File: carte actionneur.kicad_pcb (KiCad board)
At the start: 2 copper layers, 108 x 138 mm, 88 parts, among them J1 Conn_01x03_Pin, J10 Conn_01x03_Pin, J11 Conn_01x02, J12 Conn_01x02_Pin, J13 Conn_01x02_Pin, J14 Conn_01x02_Pin, J15 Conn_01x02, J16 Conn_01x02_Pin, J17 Conn_01x04_Pin, J18 Conn_01x02_Pin, J19 Conn_01x04_Pin, J2 Conn_01x02, J20 Conn_01x02_Pin, J21 Conn_01x08_Pin, J22 Conn_01x02_Pin, J23 Conn_01x02_Pin, J24 Conn_01x02_Pin, J25 Conn_01x03_Pin, J26 Conn_01x03_Pin, J27 Conn_01x03_Pin, J28 Conn_01x02_Pin, J3 Conn_01x04_Pin, J4 Conn_01x02_Pin, J5 Connecteur Programmation, J6 Conn_01x08_Pin, J7 Conn_01x03_Pin, J8 Conn_01x03_Pin, J9 Conn_01x03_Pin, Q1 Q_NMOS_GDS, Q2 QM6006D, Q3 QM6006D, Q4 QM6006D, U1 MEGA_PRO_EMBED_CH340G___ATMEG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, U2 YAAJ_DCDC_StepDown_LM2596, U3 ZXBM5210-SP, U4 YAAJ_DCDC_StepDown_LM2596, U5 YAAJ_DCDC_StepDown_LM2596, U7 ZXBM5210-SP

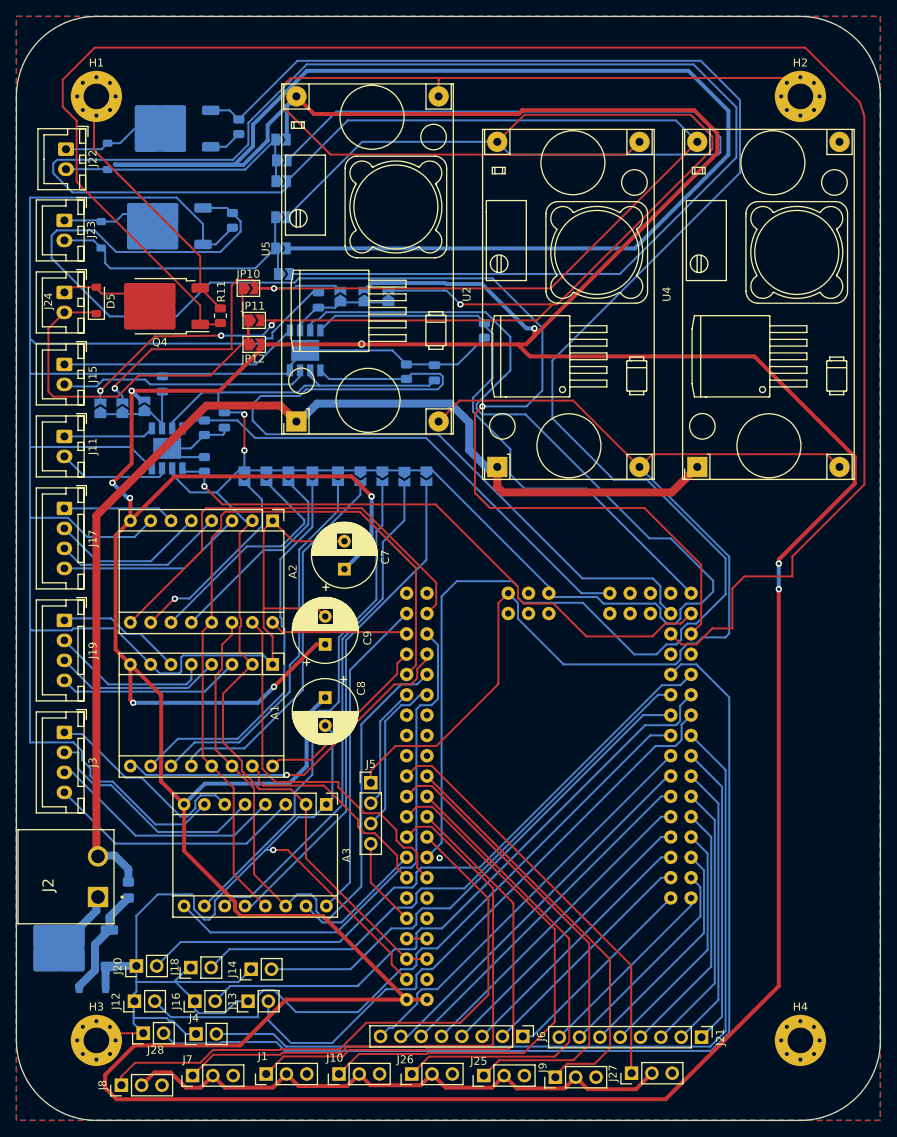
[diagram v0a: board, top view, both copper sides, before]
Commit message: Updated Arduino for 2025 (#1)
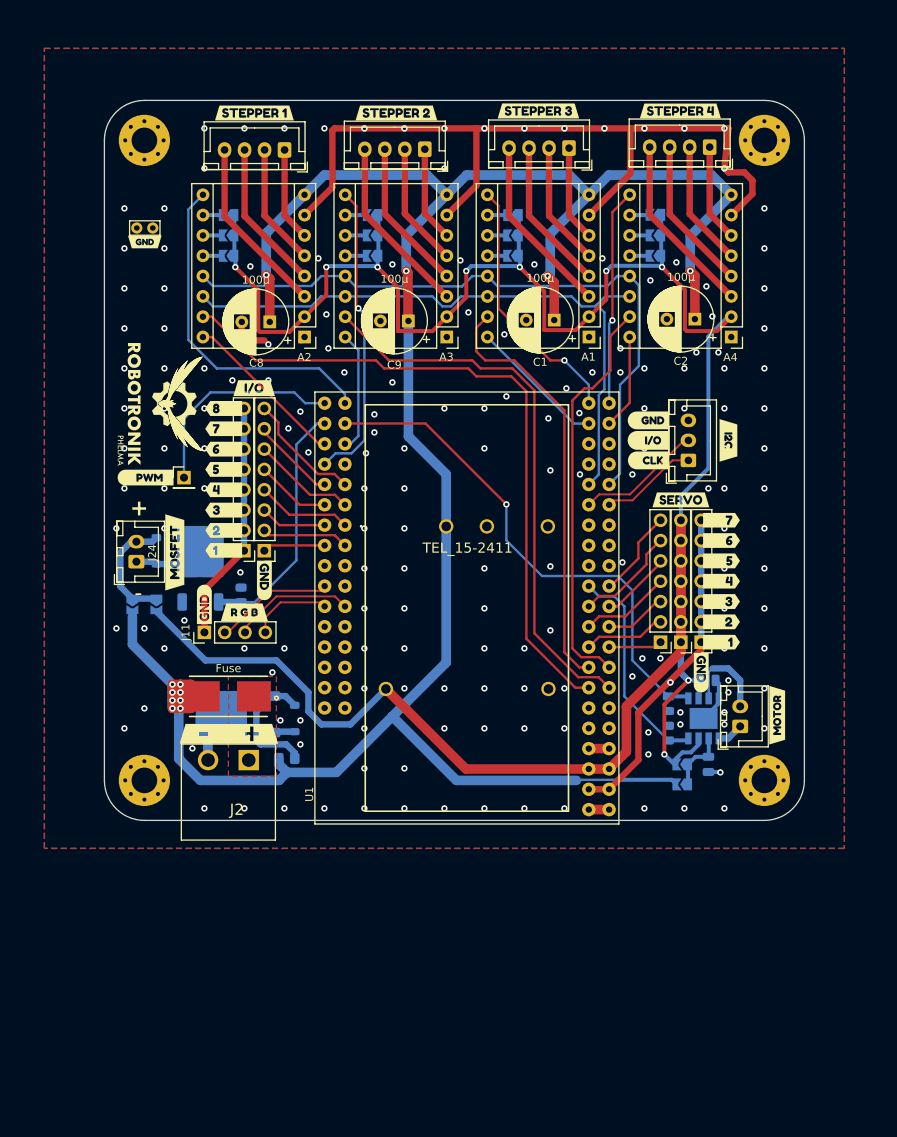
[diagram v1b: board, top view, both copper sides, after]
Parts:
- removed C3, C4: 100nF, Capacitor_SMD:C_0805_2012Metric
- removed C7: 100µ, Capacitor_THT:CP_Radial_D8.0mm_P3.50mm
- removed D3, D4: D, Diode_SMD:D_SOD-123
- removed J10, J25, J26, J27: Conn_01x03_Pin, Connector_PinHeader_2.54mm:PinHeader_1x03_P2.54mm_Vertical
- removed J12, J13, J14, J16, J18, J20, J28: Conn_01x02_Pin, Connector_PinHeader_2.54mm:PinHeader_1x02_P2.54mm_Vertical
- removed J21: Conn_01x08_Pin, Connector_PinHeader_2.54mm:PinHeader_1x08_P2.54mm_Vertical
- removed J23: Conn_01x02_Pin, Connector_JST:JST_XH_B2B-XH-A_1x02_P2.50mm_Vertical
- removed JP10, JP16, JP17, JP18, JP19, JP20, JP21, JP22: Jumper_2_Open, Jumper:SolderJumper-2_P1.3mm_Open_TrianglePad1.0x1.5mm
- removed Q2, Q3: QM6006D, Package_TO_SOT_SMD:TO-252-2
- removed R10, R9: 100k, Resistor_SMD:R_0805_2012Metric
- removed R4, R5: 10k, Resistor_SMD:R_0805_2012Metric
- removed U2, U4, U5: YAAJ_DCDC_StepDown_LM2596, lm2596:YAAJ_DCDC_StepDown_LM2596
- removed U3: ZXBM5210-SP, Package_SO:Diodes_SO-8EP
- added A4: Pololu_Breakout_A4988, A4988:Pololu_Breakout-16_15.2x20.3mm, F.Cu at (190.4, 79.1)
- added C1: 100µ, Capacitor_THT:CP_Radial_D8.0mm_P3.50mm, F.Cu at (168.2, 77.0)
- added C2: 100µ, Capacitor_THT:CP_Radial_D8.0mm_P3.50mm, F.Cu at (185.8, 76.8)
- added F1: Fuse, FuseHolder:FUSE_0154004.DR, F.Cu at (127.5, 124.0)
- added PS1: TEL_15-2411, TEL_15-2411:TEL151211, F.Cu at (154.7, 102.8)
- added REF**: LOGO, Silkscreen:LOGO, F.Cu at (113.4, 87.7)
- added REF**: Microsteps, Silkscreen:Microsteps, B.Cu at (158.7, 96.8)
- added REF**: LOGO, Silkscreen:LOGO, B.Cu at (155.2, 135.8)
- added TP1: TestPoint, TestPoint:TestPoint_Bridge_Pitch2.0mm_Drill0.7mm, F.Cu at (116.0, 65.5)
- added kibuzzard-679EA1D9: G***, kibuzzard-679EA1D9, F.Cu at (189.1, 117.2)
- added kibuzzard-679EA1F0: G***, kibuzzard-679EA1F0, F.Cu at (189.1, 114.7)
- added kibuzzard-679EA1FA: G***, kibuzzard-679EA1FA, F.Cu at (189.1, 109.6)
- added kibuzzard-679EA204: G***, kibuzzard-679EA204, F.Cu at (189.1, 107.1)
- added kibuzzard-679EA208: G***, kibuzzard-679EA208, F.Cu at (189.1, 112.1)
- added kibuzzard-679EA20F: G***, kibuzzard-679EA20F, F.Cu at (189.1, 104.5)
- added kibuzzard-679EA213: G***, kibuzzard-679EA213, F.Cu at (189.1, 102.0)
- added kibuzzard-679EA236: G***, kibuzzard-679EA236, F.Cu at (132.0, 109.5)
- added kibuzzard-679EA236: G***, kibuzzard-679EA236, F.Cu at (124.5, 112.5)
- added kibuzzard-679EA236: G***, kibuzzard-679EA236, F.Cu at (186.6, 121.0)
- added kibuzzard-679EA25C: G***, kibuzzard-679EA25C, F.Cu at (184.1, 99.4)
- added kibuzzard-679FD2F5: G***, kibuzzard-679FD2F5, B.Cu at (130.5, 58.8)
- added kibuzzard-679FD326: G***, kibuzzard-679FD326, B.Cu at (148.5, 58.8)
- added kibuzzard-679FD32C: G***, kibuzzard-679FD32C, B.Cu at (166.0, 58.8)
- added kibuzzard-679FD331: G***, kibuzzard-679FD331, B.Cu at (184.0, 58.8)
- added kibuzzard-679FD606: G***, kibuzzard-679FD606, F.Cu at (126.9, 105.8)
- added kibuzzard-679FD637: G***, kibuzzard-679FD637, F.Cu at (126.9, 103.2)
- added kibuzzard-679FD63B: G***, kibuzzard-679FD63B, F.Cu at (126.9, 100.7)
- added kibuzzard-679FD63E: G***, kibuzzard-679FD63E, F.Cu at (126.9, 98.2)
- added kibuzzard-679FD642: G***, kibuzzard-679FD642, F.Cu at (126.9, 95.6)
- added kibuzzard-679FD645: G***, kibuzzard-679FD645, F.Cu at (126.9, 93.1)
- added kibuzzard-679FD648: G***, kibuzzard-679FD648, F.Cu at (126.9, 90.5)
- added kibuzzard-679FD64B: G***, kibuzzard-679FD64B, F.Cu at (126.9, 88.0)
- added kibuzzard-679FD690: G***, kibuzzard-679FD690, F.Cu at (130.7, 85.5)
- added kibuzzard-679FD879: G***, kibuzzard-679FD879, B.Cu at (180.0, 135.0)
- added kibuzzard-679FD879: G***, kibuzzard-679FD879, B.Cu at (115.5, 116.8)
- added kibuzzard-679FD896: G***, kibuzzard-679FD896, B.Cu at (118.5, 116.3)
- added kibuzzard-679FD896: G***, kibuzzard-679FD896, B.Cu at (180.5, 132.5)
- added kibuzzard-679FDC70: G***, kibuzzard-679FDC70, F.Cu at (130.8, 51.1)
- added kibuzzard-679FDCB9: G***, kibuzzard-679FDCB9, F.Cu at (148.5, 51.1)
- added kibuzzard-679FDCBD: G***, kibuzzard-679FDCBD, F.Cu at (166.3, 50.8)
- added kibuzzard-679FDCC2: G***, kibuzzard-679FDCC2, F.Cu at (184.0, 50.8)
- added kibuzzard-67A0E12F: G***, kibuzzard-67A0E12F, F.Cu at (129.5, 113.5)
- added kibuzzard-67A0F0A3: G***, kibuzzard-67A0F0A3, F.Cu at (190.0, 92.0)
- added kibuzzard-67A0F0D2: G***, kibuzzard-67A0F0D2, F.Cu at (180.0, 89.5)
- added kibuzzard-67A0F0E8: G***, kibuzzard-67A0F0E8, F.Cu at (180.0, 92.0)
- added kibuzzard-67A0F0EE: G***, kibuzzard-67A0F0EE, F.Cu at (180.0, 94.5)
- added kibuzzard-67A13B87: G***, kibuzzard-67A13B87, F.Cu at (127.6, 128.7)
- added kibuzzard-67A14542: G***, kibuzzard-67A14542, F.Cu at (117.0, 67.2)
- added kibuzzard-67A145CB: G***, kibuzzard-67A145CB, F.Cu at (120.8, 106.0)
- added kibuzzard-67A1464C: G***, kibuzzard-67A1464C, F.Cu at (196.1, 126.3)
- added kibuzzard-67A14A78: G***, kibuzzard-67A14A78, F.Cu at (117.2, 96.7)
- D5, JP11, JP12, Q4, R11: moved to B.Cu
- J1: value Conn_01x03_Pin -> Conn_01x08_Pin; footprint Connector_PinHeader_2.54mm:PinHeader_1x03_P2.54mm_Vertical -> Connector_PinHeader_2.54mm:PinHeader_1x08_P2.54mm_Vertical
- J11: value Conn_01x02 -> Conn_01x04_Pin; footprint Connector_JST:JST_XH_B2B-XH-A_1x02_P2.50mm_Vertical -> Connector_PinHeader_2.54mm:PinHeader_1x04_P2.54mm_Vertical
- J22: value Conn_01x02_Pin -> Conn_01x04_Pin; footprint Connector_JST:JST_XH_B2B-XH-A_1x02_P2.50mm_Vertical -> Connector_JST:JST_XH_B4B-XH-A_1x04_P2.50mm_Vertical
- J4: value Conn_01x02_Pin -> Conn_01x08_Pin; footprint Connector_PinHeader_2.54mm:PinHeader_1x02_P2.54mm_Vertical -> Connector_PinHeader_2.54mm:PinHeader_1x08_P2.54mm_Vertical
- J5: value Connecteur Programmation -> Conn_01x03; footprint Connector_PinHeader_2.54mm:PinHeader_1x04_P2.54mm_Vertical -> Connector_JST:JST_XH_B3B-XH-A_1x03_P2.50mm_Vertical
- J6: value Conn_01x08_Pin -> Conn_01x07_Pin; footprint Connector_PinHeader_2.54mm:PinHeader_1x08_P2.54mm_Vertical -> Connector_PinHeader_2.54mm:PinHeader_1x07_P2.54mm_Vertical
- J7, J8: value Conn_01x03_Pin -> Conn_01x07_Pin; footprint Connector_PinHeader_2.54mm:PinHeader_1x03_P2.54mm_Vertical -> Connector_PinHeader_2.54mm:PinHeader_1x07_P2.54mm_Vertical
- J9: value Conn_01x03_Pin -> Conn_01x01_Pin; footprint Connector_PinHeader_2.54mm:PinHeader_1x03_P2.54mm_Vertical -> Connector_PinHeader_2.54mm:PinHeader_1x01_P2.54mm_Vertical
- U1: moved to F.Cu
- moved J15 95.8 mm to (191.5, 127.8), turned to 90 degrees
- moved J8 91.2 mm to (186.6, 117.2), turned to 180 degrees
- moved J9 88.2 mm to (122.0, 96.7), turned to 0 degrees
- moved J19 86.4 mm to (170.1, 55.5), turned to 180 degrees
- moved J3 85.7 mm to (152.1, 55.6), turned to 180 degrees
- moved J7 81.6 mm to (184.1, 117.2), turned to 180 degrees
- moved J22 80.5 mm to (187.7, 55.3), turned to 180 degrees
- moved C6 75.8 mm to (187.5, 132.5), turned to -90 degrees
- moved JP24 72.8 mm to (184.2, 135.0), turned to 180 degrees
- moved JP23 69.1 mm to (184.2, 132.5), turned to 180 degrees
- moved U7 67.8 mm to (186.9, 126.8), turned to 90 degrees
- moved J1 65.4 mm to (132.0, 105.8), turned to 180 degrees
- moved J4 60.7 mm to (129.4, 105.8), turned to 180 degrees
- moved A3 60.3 mm to (154.8, 79.1), turned to 180 degrees
- moved A1 56.9 mm to (172.6, 79.1), turned to 180 degrees
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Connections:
- A1 pad 15: STEP1 -> STEP3
- A1 pad 16: DIR1 -> DIR3
- A1 pad 8: 12V Mot -> +BATT
- A2 pad 15: STEP2 -> STEP1
- A2 pad 16: DIR2 -> DIR1
- A2 pad 8: 12V Mot -> +BATT
- A3 pad 15: STEP3 -> STEP2
- A3 pad 16: DIR3 -> DIR2
- A3 pad 8: 12V Mot -> +BATT
- C8 pad 1: 12V Mot -> +BATT
- C9 pad 1: 12V Mot -> +BATT
- J1 pad 1: Servo4 -> Sens1
- J1 pad 2: 5VServo -> Sens2
- J1 pad 3: GND -> Sens3
- J11 pad 1: Net-(J11-Pin_1) -> GND
- J11 pad 2: Net-(J11-Pin_2) -> LED_R
- J2 pad 2: +24V -> Net-(J2-Pin_2)
- J4 pad 2: Capt1 -> GND
- J5 pad 1: GND -> SWCLK
- J5 pad 2: SWCLK -> SWDIO
- J5 pad 3: SWDIO -> GND
- J6 pad 1: Net-(J6-Pin_1) -> Servo1
- J6 pad 2: Net-(J6-Pin_2) -> Servo2
- J6 pad 3: Net-(J6-Pin_3) -> Servo3
- J6 pad 4: Net-(J6-Pin_4) -> Servo4
- J6 pad 5: Net-(J6-Pin_5) -> Servo5
- J6 pad 6: Net-(J6-Pin_6) -> Servo6
- J6 pad 7: Net-(J6-Pin_7) -> Servo7
- J7 pad 1: Servo1 -> +5V
- J7 pad 2: 5VServo -> +5V
- J7 pad 3: GND -> +5V
- J8 pad 1: Servo2 -> GND
- J8 pad 2: 5VServo -> GND
- J9 pad 1: Servo8 -> PWM_LIDAR
- JP11 pad 2: 5V Servo -> +5V
- JP12 pad 2: 12V Mot -> +BATT
- JP13 pad 1: Net-(D4-K) -> +5V
- JP13 pad 2: VmotDC -> Net-(A4-MS1)
- JP14 pad 1: Net-(D4-K) -> +5V
- JP14 pad 2: 5V Servo -> Net-(A4-MS2)
- JP15 pad 1: Net-(D4-K) -> +5V
- JP15 pad 2: 12V Mot -> Net-(A4-MS3)
- JP23 pad 2: 5V Servo -> +5V
- JP24 pad 2: 12V Mot -> +BATT
- Q1 pad 2: Net-(J2-Pin_1) -> Net-(J2-Pin_2)
- Q4 pad 1: ctrlActionneur3 -> ctrlActionneur1
- R1 pad 1: +24V -> +BATT
- R11 pad 1: ctrlActionneur3 -> ctrlActionneur1
- U1 pad 3V3_1: +3.3V -> unconnected-(U1-3V3-Pad3V3_1)
- U1 pad 3V3_2: +3.3V -> unconnected-(U1-3V3-Pad3V3_1)
- U1 pad A0: Net-(J21-Pin_8) -> unconnected-(U1-PadA0)
- U1 pad A1: Net-(J6-Pin_1) -> unconnected-(U1-PadA1)
- U1 pad A10: Net-(J21-Pin_3) -> LED_B
- U1 pad A11: Net-(J6-Pin_6) -> LED_G
- U1 pad A12: Net-(J21-Pin_2) -> LED_R
- U1 pad A13: Net-(J6-Pin_7) -> unconnected-(U1-PadA13)
- U1 pad A14: Net-(J21-Pin_1) -> unconnected-(U1-PadA14)
- U1 pad A15: Net-(J6-Pin_8) -> unconnected-(U1-PadA15)
- U1 pad A2: Net-(J21-Pin_7) -> unconnected-(U1-PadA2)
- U1 pad A3: Net-(J6-Pin_2) -> unconnected-(U1-PadA3)
- U1 pad A4: Net-(J21-Pin_6) -> unconnected-(U1-PadA4)
- U1 pad A5: Net-(J6-Pin_3) -> unconnected-(U1-PadA5)
- U1 pad A6: Net-(J21-Pin_5) -> unconnected-(U1-PadA6)
- U1 pad A7: Net-(J6-Pin_4) -> unconnected-(U1-PadA7)
- U1 pad A8: Net-(J21-Pin_4) -> unconnected-(U1-PadA8)
- U1 pad A9: Net-(J6-Pin_5) -> unconnected-(U1-PadA9)
- U1 pad D12: Servo8 -> FWD1
- U1 pad D2: STEP2 -> STEP1
- U1 pad D24: Enable3 -> unconnected-(U1-PadD24)
- U1 pad D25: DIR1 -> unconnected-(U1-PadD25)
- U1 pad D26: Enable2 -> unconnected-(U1-PadD26)
- U1 pad D27: DIR2 -> unconnected-(U1-PadD27)
- U1 pad D28: Enable1 -> DIR3
- U1 pad D29: DIR3 -> DIR4
- U1 pad D3: STEP1 -> STEP2
- U1 pad D30: unconnected-(U1-PadD30) -> Enable3
- U1 pad D31: unconnected-(U1-PadD31) -> Enable4
- U1 pad D32: Capt1 -> Sens1
- U1 pad D33: Capt2 -> Sens2
- U1 pad D34: Capt3 -> Sens3
- U1 pad D35: Capt4 -> Sens4
- U1 pad D36: Capt5 -> Sens5
- U1 pad D37: Capt6 -> Sens6
- U1 pad D38: Capt7 -> Sens7
- U1 pad D39: Capt8 -> Sens8
- U1 pad D4: ctrlActionneur1 -> STEP3
- U1 pad D40: unconnected-(U1-PadD40) -> Enable2
- U1 pad D42: ctrlActionneur2 -> DIR1
- U1 pad D43: ctrlActionneur3 -> DIR2
- U1 pad D44: REV2 -> ctrlActionneur1
- U1 pad D46: FWD1 -> PWM_LIDAR
- U1 pad D47: unconnected-(U1-PadD47) -> Enable1
- U1 pad D5: STEP3 -> STEP4
- U1 pad RST: Net-(J5-Pin_4) -> unconnected-(U1-PadRST)
- U1 pad VIN_1: 12V Mot -> unconnected-(U1-VIN-PadVIN_1)
- U1 pad VIN_2: 12V Mot -> unconnected-(U1-VIN-PadVIN_1)
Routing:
- net 12V Mot: track 812.7 -> 0.00 mm, vias 9 -> 0
- net GND: track 791.3 -> 187.9 mm, vias 2 -> 180
- net VmotDC: track 355.5 -> 0.00 mm, vias 2 -> 0
- net +BATT: track 0.00 -> 302.4 mm, vias 0 -> 12
- net 5V Servo: track 263.3 -> 0.00 mm, vias 4 -> 0
- net ctrlActionneur3: track 229.6 -> 0.00 mm
- net ctrlActionneur1: track 232.8 -> 31.0 mm
- net ctrlActionneur2: track 173.0 -> 0.00 mm, vias 1 -> 0
- net +24V: track 141.5 -> 0.00 mm
- net Capt8: track 124.2 -> 0.00 mm
- net Capt1: track 103.9 -> 0.00 mm
- net Capt2: track 84.6 -> 0.00 mm
- net Capt7: track 82.7 -> 0.00 mm
- net Capt5: track 77.7 -> 0.00 mm
- net Capt3: track 75.4 -> 0.00 mm
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- added copper zone on F.Cu, net Net-(J2-Pin_1)
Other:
- board size 108 x 138 mm -> 87.5 x 90 mm
- board text added: "+"
- board text added: "-"
- board text added: "Carte Actionneurs Arduino Ludovic Bouchard Rev1 02/2025"
- board text added: "MS1"
- board text added: "MS2"
- board text added: "MS3"
